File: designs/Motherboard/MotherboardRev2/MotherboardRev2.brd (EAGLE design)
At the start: 160 x 100 mm, 142 parts, among them IC1 PIC24FJ64GB202, IC3 PIC24FJ64GB202, Q1 BSS123, Q2 BSS123, Q3 BSS123, Q4 BSS123, U1 LMS8117AMP-3.3, U3 LMS8117AMP-3.3

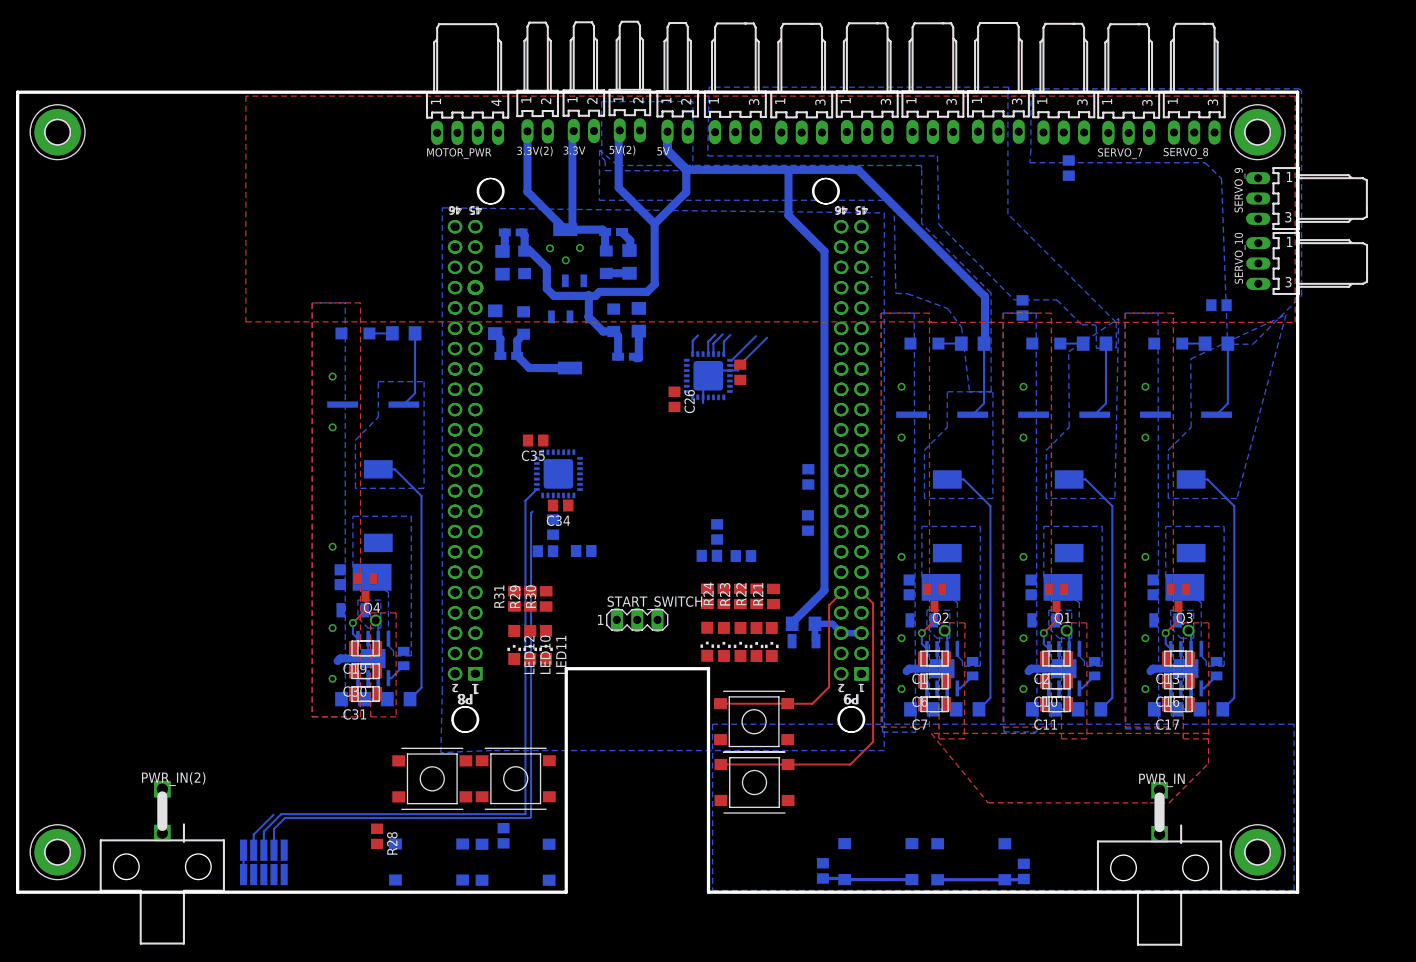
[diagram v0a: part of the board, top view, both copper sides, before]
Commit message: Final Motherboard
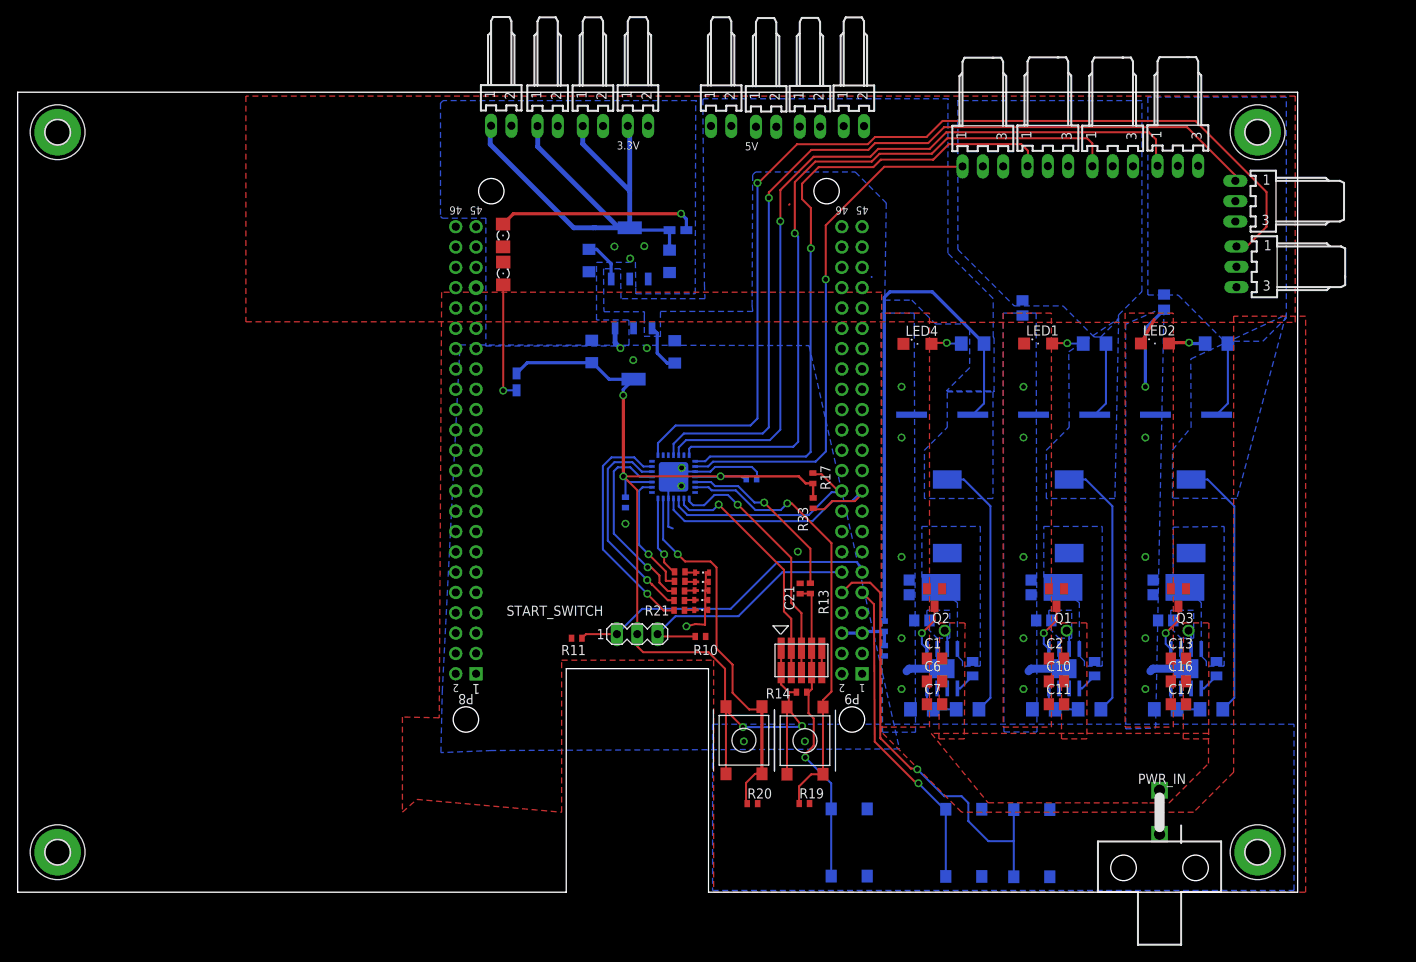
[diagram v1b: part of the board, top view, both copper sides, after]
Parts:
- removed C19, C30, C31, C32: 4.7uF, 5v:1206
- removed C20: 10nF, 5v:0805
- removed C22: 330uF, 5v:SM_RADIAL_10AMM
- removed C33: 10uF, rcl:C0805
- removed C34, C35, C36: .1uF, rcl:C0805
- removed D4: PDS760-13, 5v:POWERDI5
- removed D6, D8: 6V_Pwr, SparkFun-LED:FKIT-LED-1206
- removed IC1: PIC24FJ64GB202, microchip:QFN28-ML_6X6MM
- removed L4: (no value), WE-HCC:WE-HCC_1090
- removed LED10, LED11, LED12: (no value), motherboard_i_autoroute:LED_CHIPLED_1206
- removed LED3: (no value), led:SML1206
- removed MOTOR_PWR: (no value), Son_of_Dark_Powersch:7395-04
- removed PWR_IN(2): (no value), Son_of_Dark_Powersch:5569-2
- removed Q4: BSS123, transistor-small-signal:SOT23
- removed R12: 10k, rcl:R1206
- removed R16, R35: (no value), rcl:R0805W
- removed R18: 470, rcl:R0805
- removed R26: 10k, rcl:R0805
- removed R27, R28: 4.7k, rcl:R0805
- removed R29, R30, R31: (no value), rcl:M0805
- removed SERVO_10, SERVO_7, SERVO_8, SERVO_9: (no value), con-molex:7395-03
- removed U$10: Switch3, Parts4Class:MC32882_FINAL
- removed U$11: Switch1, Parts4Class:MC32882_FINAL
- removed U$12: Switch2, Parts4Class:MC32882_FINAL
- removed U$3: BEAGLE_BONE_BLACK_CAPE, SparkFun-Boards:BEAGLE_BONE_BLACK_CAPE
- removed U$9: TPS5450DDAR, 5v:R-PDSO-G8
- added 3.3V(2)1, 3.3V1, 5V(2)1, 5V1: (no value), Son_of_Dark_Powersch:7395-02
- C1, C10, C11, C12, C13, C16, C17, C18, C2, C6, C7, C8: device 5v:1206 -> rcl:C0805
- C21, C25, C26: device rcl:C0805 -> rcl:C0402
- C37: device 3-3_fixed:1206 -> rcl:C0402
- LED5, LED6, LED7, LED8, LED9: device motherboard_i_autoroute:LED_CHIPLED_1206 -> led:CHIPLED-0603-TTW
- R10: value 10k -> (none); device rcl:R1206 -> rcl:R0402
- R11, R32: device rcl:R1206 -> rcl:R0402
- R13, R14, R17, R19, R20, R33: device rcl:R0805 -> rcl:R0402
- R21, R22, R23, R24, R25: device rcl:M0805 -> rcl:R0402
- moved PROGRAMMING 71.8 mm to (98.0, 29.0), flipped to the top
- moved SERVO_1 64.9 mm to (152.4, 78.2), turned to 90 degrees
- moved SERVO_2 54.9 mm to (152.2, 86.4), turned to 90 degrees
- moved U$5 52.7 mm to (103.9, 6.21), flipped to the bottom, turned to 270 degrees
- moved SERVO_3 39.1 mm to (145.0, 90.8)
- moved R10 38.5 mm to (85.3, 32.0), flipped to the top
- moved U$14 37.9 mm to (126.8, 6.13), flipped to the bottom, turned to 270 degrees
- moved R20 35.0 mm to (91.8, 11.1), flipped to the top, turned to 0 degrees
- moved U$7 32.2 mm to (90.8, 19.0), flipped to the top, turned to 270 degrees
- moved R11 29.0 mm to (69.9, 31.8), flipped to the top, turned to 0 degrees
- moved U$13 27.2 mm to (118.3, 6.17), flipped to the bottom, turned to 270 degrees
- moved SERVO_4 22.9 mm to (136.9, 90.7)
- moved R14 20.6 mm to (98.0, 25.0), flipped to the top, turned to 180 degrees
- moved U$6 17.7 mm to (98.4, 18.9), flipped to the top, turned to 270 degrees
- moved D7 16.1 mm to (60.7, 82.1), flipped to the top
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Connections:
- removed net BOOT4: C20.1, U$9.1
- removed net EN4: Q4.1
- removed net ENA_4: Q4.3, U$9.5
- removed net IO3(1): IC1.7, R29.2
- removed net IO4(1): IC1.9, R30.2
- removed net IO5(1): IC1.11, R31.2
- removed net MCLR'(1): IC1.26, R18.1
- removed net MCLR(1): C36.1, R18.2, R26.1, U$10.P$2, U$10.P$3
- removed net N$12: U$3.P8.7
- removed net N$13: D6.A, R16.1
- removed net N$14: U$3.P8.8
- removed net N$15: LED10.A, R29.1
- removed net N$16: LED11.A, R30.1
- removed net N$17: LED12.A, R31.1
- removed net N$21: D8.A, R35.1
- removed net N$4: LED3.A, R12.1
- removed net OC1(1): IC1.23, SERVO_9.1
- removed net OC2(1): IC1.22, SERVO_8.1
- removed net OC3(1): IC1.21, SERVO_10.1
- removed net OC4(1): IC1.19, SERVO_7.1
- removed net PH4: C20.2, D4.3, L4.1, U$9.8
- removed net SWITCH_3: IC1.6, R27.1, U$11.P$2, U$11.P$3
- removed net SWITCH_4: IC1.27, R28.1, U$12.P$2, U$12.P$3
- removed net VOUT4: C22.1, L4.2, MOTOR_PWR.2, MOTOR_PWR.3, R10.2, R12.2
- removed net VSNS4: R10.1, R11.2, U$9.4
- net 3.3V: no longer C34.1, C35.1, IC1.10, IC1.25, R26.2, U$11.P$1, U$11.P$4, U$12.P$1, U$12.P$4
- net GND: now also 3.3V(2)1.2, 3.3V1.2, 5V(2)1.2, 5V1.2, LED5.C@1, LED6.C@1, LED7.C@1, LED8.C@1, LED9.C@1, R10.1; no longer C19.1, C22.2, C30.1, C31.1, C32.1, C33.2, C34.2, C35.2, C36.2, D4.1, D6.C, D8.C, IC1.24, IC1.5, LED10.C, LED11.C, LED12.C, LED3.C, LED5.C, LED6.C, LED7.C, LED8.C, LED9.C, MOTOR_PWR.1, MOTOR_PWR.4, PWR_IN(2).1, Q4.2, R27.2, R28.2, SERVO_10.3, SERVO_7.3, SERVO_8.3, SERVO_9.3, U$10.P$1, U$10.P$4, U$3.P8.1, U$3.P8.2, U$3.P9.1, U$3.P9.2, U$3.P9.43, U$3.P9.44, U$3.P9.45, U$3.P9.46, U$9.6, U$9.9
- net IO3: now also R25.2; no longer R21.2
- net IO4: now also R24.2; no longer R25.2
- net IO5: now also R23.2; no longer R24.2
- net IO7: now also R21.2; no longer R23.2
- net IO8: no longer IC1.28
- net N$5: now also LED5.A@1; no longer LED5.A
- net N$6: now also LED6.A@1; no longer LED6.A
- net N$7: now also LED7.A@1; no longer LED7.A
- net N$8: now also LED8.A@1; no longer LED8.A
- net N$9: now also LED9.A@1; no longer LED9.A
- net OC1: now also SERVO_6.1; no longer SERVO_1.1
- net OC2: now also SERVO_5.1; no longer SERVO_2.1
- net OC3: now also SERVO_4.1; no longer SERVO_3.1
- net OC4: now also SERVO_3.1; no longer SERVO_4.1
- net OC5: now also SERVO_2.1; no longer SERVO_5.1
- net OC6: now also SERVO_1.1; no longer SERVO_6.1
- net PGC1: no longer IC1.2
- net PGD1: no longer IC1.1
- net SCL: no longer IC1.4
- net SDA: no longer IC1.3
- net START_LEFT: now also R10.2
- net START_RIGHT: now also R11.2
- net VCC: no longer C19.2, C30.2, C31.2, C32.2, PWR_IN(2).2, U$9.7
- net VOUT1: now also 5V(2)1.1, 5V1.1; no longer R16.2, R35.2
- net VOUT2: now also SERVO_6.2; no longer C27.1, SERVO_1.2, SERVO_2.2, SERVO_3.2
- net VOUT3: now also C27.1, SERVO_1.2, SERVO_2.2, SERVO_3.2; no longer C33.1, SERVO_10.2, SERVO_6.2, SERVO_7.2, SERVO_8.2, SERVO_9.2
- net VOUT5: now also 3.3V(2)1.1, 3.3V1.1
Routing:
- net 3.3V: track 10.3 -> 145.3 mm, vias 0 -> 5
- net OC6: track 2.63 -> 124.3 mm, vias 0 -> 1
- net VOUT1: track 226.0 -> 109.9 mm
- net OC5: track 2.83 -> 108.5 mm, vias 0 -> 1
- net OC4: track 2.97 -> 98.2 mm, vias 0 -> 1
- net OC3: track 2.74 -> 90.0 mm, vias 0 -> 1
- net OC2: track 4.50 -> 81.5 mm, vias 0 -> 1
- net OC1: track 6.11 -> 65.6 mm, vias 0 -> 1
- net PGD1: track 77.1 -> 32.0 mm, vias 0 -> 1
- net SWITCH_1: track 11.3 -> 55.7 mm, vias 0 -> 1
- net PGC1: track 73.7 -> 30.5 mm, vias 0 -> 1
- net VOUT4: track 42.2 -> 0.00 mm
- net START_RIGHT: track 0.00 -> 39.8 mm
- net VOUT5: track 34.2 -> 73.3 mm
- net SWITCH_2: track 10.9 -> 47.9 mm, vias 0 -> 1
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- removed copper zone on layer 16, net PH4
- removed copper zone on layer 16, net VOUT4
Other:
- board text added: "BBB Power Off"
- board text added: "BBB Reset"
- board text added: "PIC Reset"
